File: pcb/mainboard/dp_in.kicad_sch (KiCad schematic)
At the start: 33 parts, among them J1 GT-USB-7007A, U16 USBLC6-2P6, U17 FUSB302BMPX, U18 CBTL02043A, U19 PTN3460

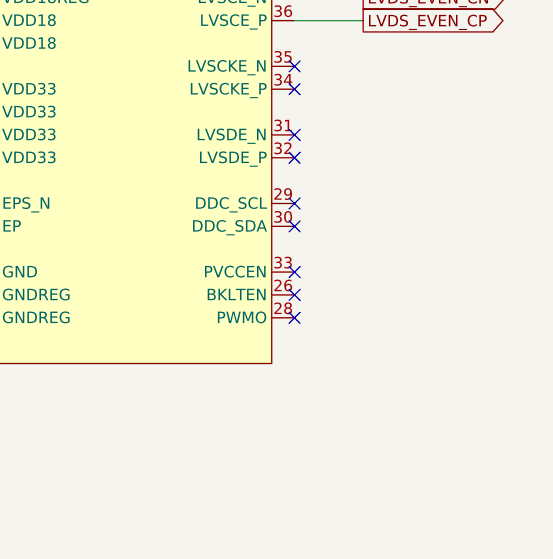
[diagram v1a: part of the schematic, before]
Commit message: Sync local PCB changes
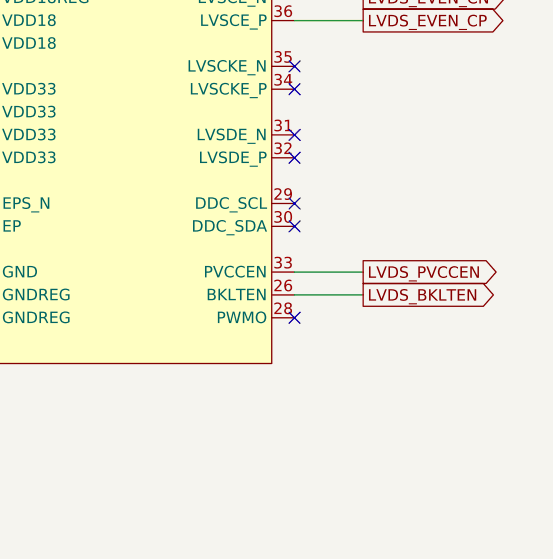
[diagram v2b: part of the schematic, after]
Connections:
- net LVDS_BKLTEN: now reaches U19.26 (BKLTEN)
- net LVDS_PVCCEN: now reaches U19.33 (PVCCEN)
- no-connect marks 17 -> 15
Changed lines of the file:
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@@
-	)
-	(no_connect
-		(at 256.54 134.62)
 	)
 	(no_connect
@@
 	)
 	(no_connect
-		(at 256.54 137.16)
-	)
-	(no_connect
 		(at 256.54 119.38)
 	)
@@
 	(wire
 		(pts
+			(xy 256.54 134.62) (xy 264.16 134.62)
+		)
+		(stroke
+			(width 0)
+			(type default)
+		)
+	)
+	(wire
+		(pts
 			(xy 195.58 78.74) (xy 220.98 78.74)
 		)
@@
 		(pts
 			(xy 101.6 58.42) (xy 106.68 58.42)
+		)
+		(stroke
+			(width 0)
+			(type default)
+		)
+	)
+	(wire
+		(pts
+			(xy 256.54 137.16) (xy 264.16 137.16)
 		)
 		(stroke
@@
 		)
 	)
+	(global_label "LVDS_PVCCEN"
+		(shape output)
+		(at 264.16 134.62 0)
+		(fields_autoplaced yes)
+		(effects
+			(font
+				(size 1.27 1.27)
+			)
+			(justify left)
+		)
+		(property "Intersheetrefs" "${INTERSHEET_REFS}"
+			(at 280.0871 134.62 0)
+			(effects
+				(font
+					(size 1.27 1.27)
+				)
+				(justify left)
+				(hide yes)
+			)
+		)
+	)
 	(global_label "LVDS_EVEN_BN"
 		(shape output)
@@
 			(effects
 				(font
+					(size 1.27 1.27)
+				)
+				(justify left)
+				(hide yes)
+			)
+		)
+	)
+	(global_label "LVDS_BKLTEN"
+		(shape output)
+		(at 264.16 137.16 0)
+		(fields_autoplaced yes)
+		(effects
+			(font
+				(size 1.27 1.27)
+			)
+			(justify left)
+		)
+		(property "Intersheetrefs" "${INTERSHEET_REFS}"
+			(at 279.7242 137.16 0)
+			(effects
+				(font
